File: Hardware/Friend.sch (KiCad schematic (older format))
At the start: 21 parts

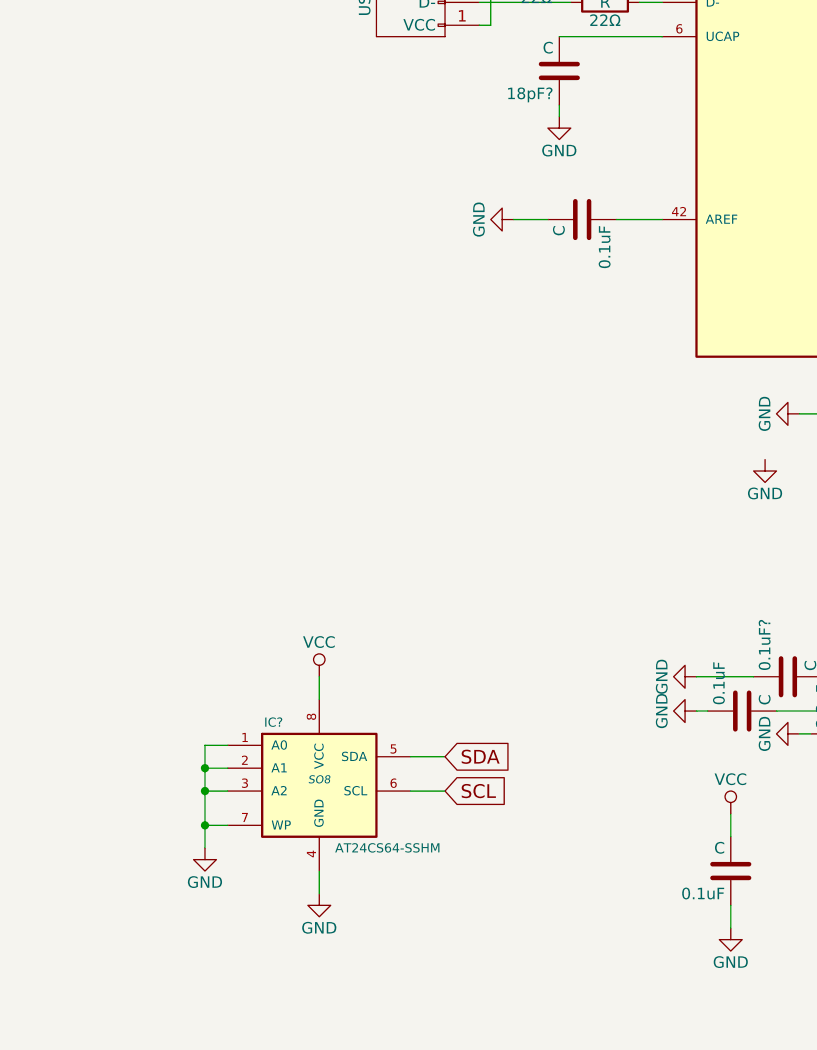
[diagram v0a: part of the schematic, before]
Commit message: dual ignition systems
one for good luck
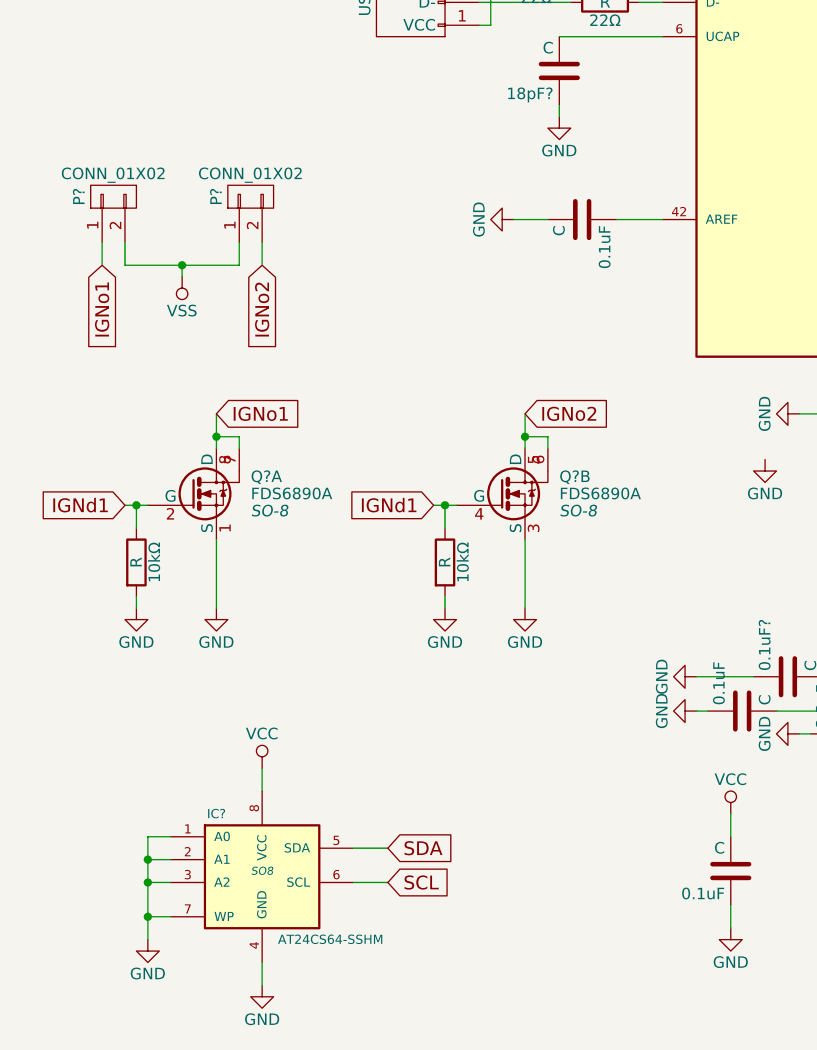
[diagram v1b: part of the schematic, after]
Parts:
- added 10kΩ (x2): R, symbol R
- added P? (x2): CONN_01X02, symbol CONN_01X02
- added Q? (x2): FDS6890A, SO-8, symbol FDS6890A
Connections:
- net GND: now also 10kΩ.2, 10kΩ.2, Q?.1 (S), Q?.3 (S)
- net VSS: now also P?.1 (P1), P?.2 (P2)
- new net IGNd1: 10kΩ.1, 10kΩ.1, Q?.2 (G), Q?.4 (G)
- new net IGNo1: P?.1 (P1), Q?.7, Q?.8 (D)
- new net IGNo2: P?.2 (P2), Q?.5 (D), Q?.6
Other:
- moved on the sheet: IC?
